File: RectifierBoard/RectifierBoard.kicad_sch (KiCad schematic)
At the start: 16 parts, among them J1 MKDS 1,5/2-7,62, J2 Standby, J3 B+ L1, J4 B+PI, J5 B+ Preamp

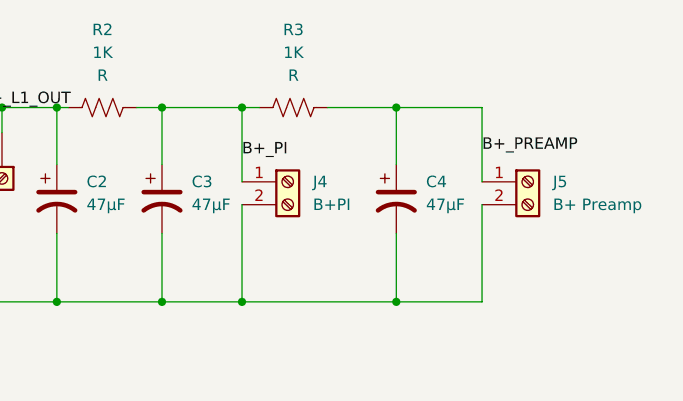
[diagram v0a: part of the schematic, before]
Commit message: Getting closer
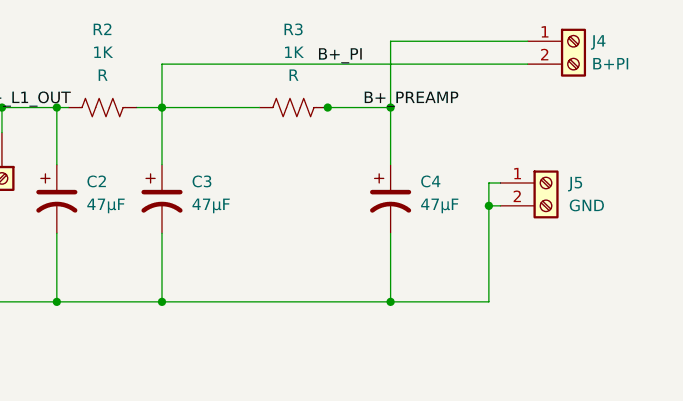
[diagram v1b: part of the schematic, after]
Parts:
- J5: value B+ Preamp -> GND
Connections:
- net B+_PI: now also J4.2 (Pin_2); no longer J4.1 (Pin_1)
- net B+_PREAMP: now also J4.1 (Pin_1); no longer J5.1 (Pin_1)
- net GND: now also J5.1 (Pin_1); no longer J4.2 (Pin_2)
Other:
- moved on the sheet: C4, J5
